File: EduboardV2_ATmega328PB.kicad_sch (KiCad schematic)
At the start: 25 parts, among them J1 EduboardV2 PCIE UP Board Conn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, SW1 K2-1102SP-C4SC-04, U2 ATMEGA328PB-AUR

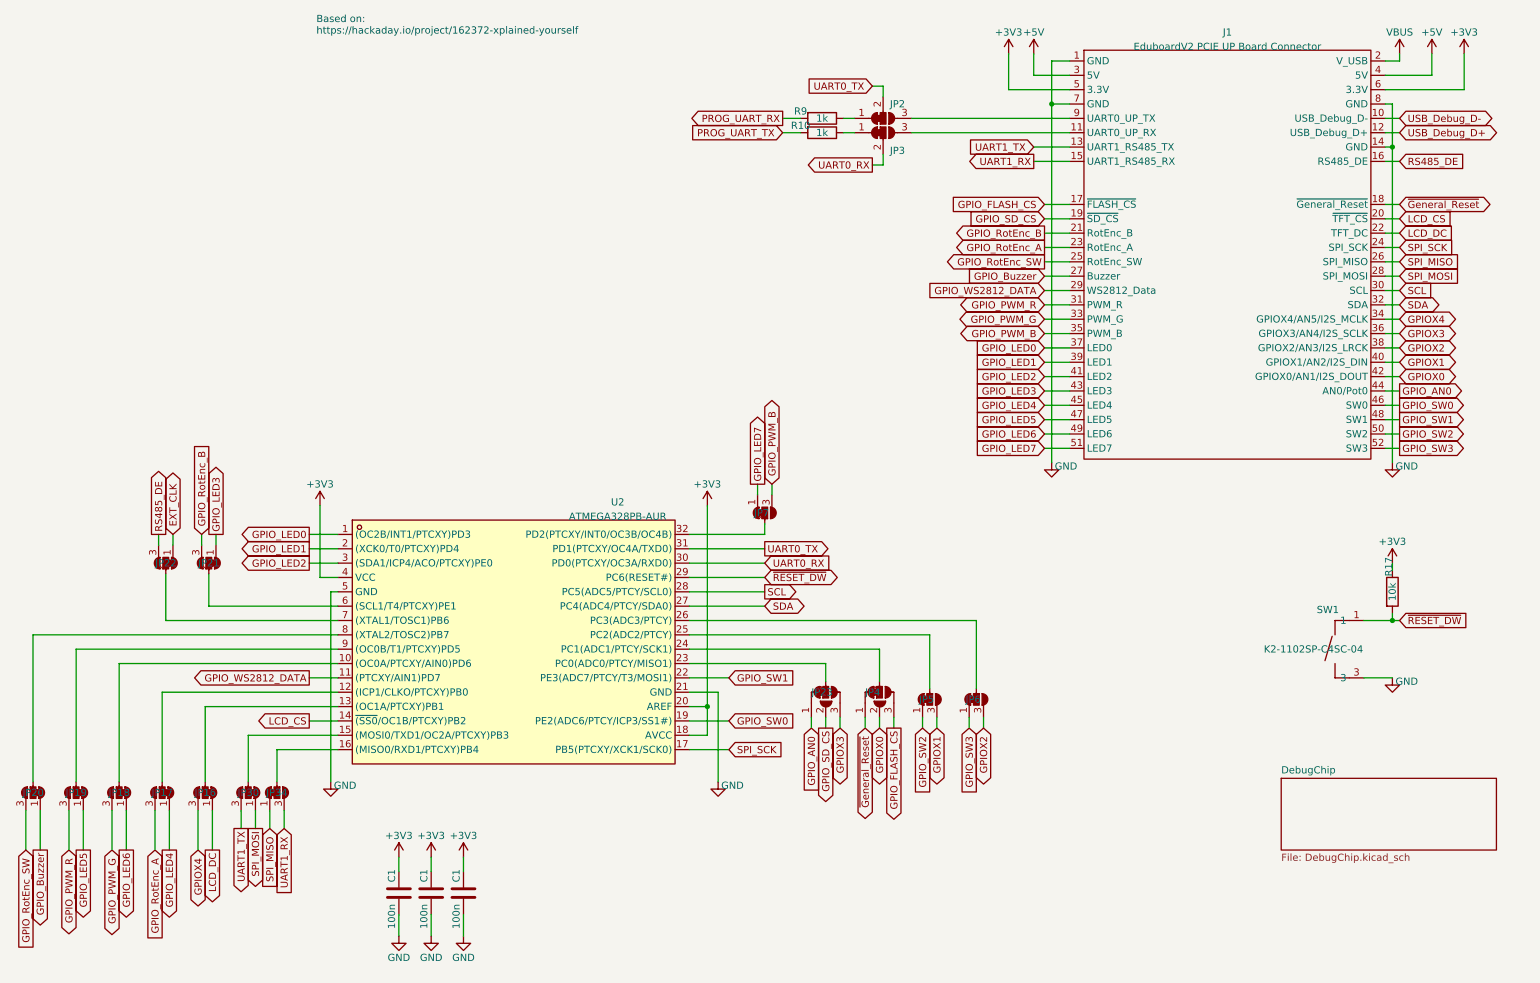
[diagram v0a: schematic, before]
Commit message: arrange parts and layout v1.1.
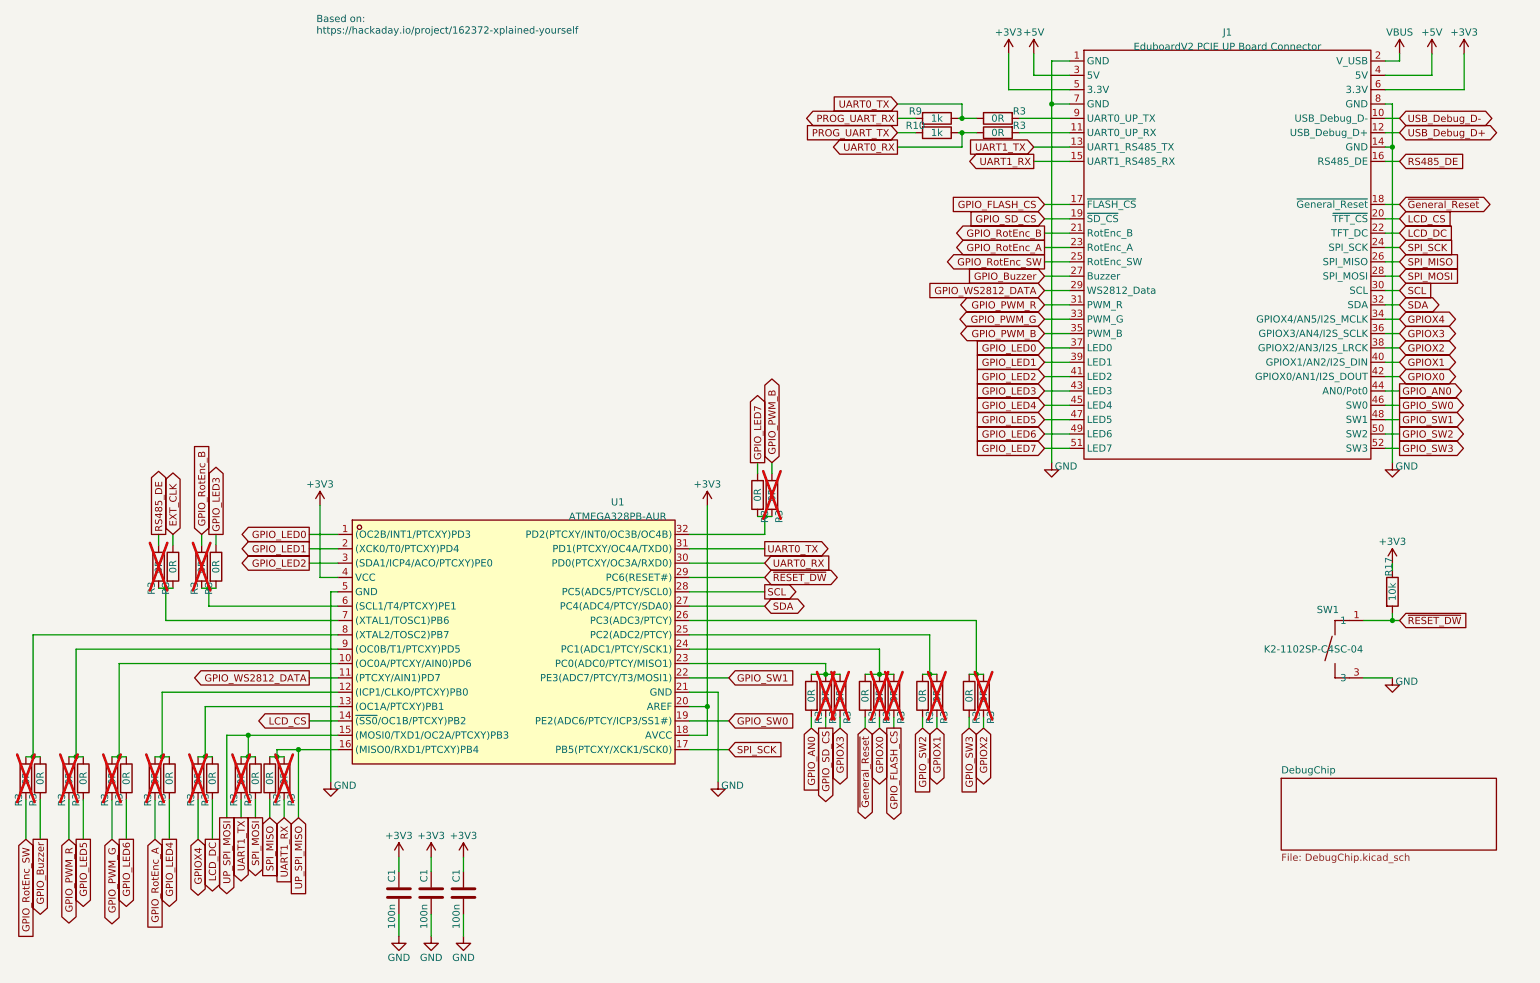
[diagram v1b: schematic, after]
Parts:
- removed JP16, JP17, JP18, JP19, JP20, JP21, JP22, JP30, JP34, JP5, JP6, JP7: SolderJumper_3_Bridged12, EduboardV2_kicadlib:SolderJumper_Small-3_bridged12, symbol EduboardV2_kicadlib:SolderJumper_Small_3_Bridged12
- removed JP2, JP3: SolderJumper_3_Bridged12, EduboardV2_kicadlib:SolderJumper_Small-3_bridged12, symbol Jumper:SolderJumper_3_Bridged12
- removed JP23, JP4: SolderJumper_3_Bridged12, EduboardV2_kicadlib:SolderJumper_Small-4_bridged14, symbol EduboardV2_kicadlib:SolderJumper_Small_4_Bridged14
- added R3 (x32): 0R, Resistor_SMD:R_0603_1608Metric, symbol Device:R
- renumbered U2 to U1
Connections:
- net EXT_CLK: now also R3.1
- net GPIOX0: now also R3.2
- net GPIOX1: now also R3.2
- net GPIOX2: now also R3.2
- net GPIOX3: now also R3.2
- net GPIOX4: now also R3.2
- net GPIO_AN0: now also R3.2
- net GPIO_Buzzer: now also R3.2
- net GPIO_FLASH_CS: now also R3.2
- net GPIO_LED3: now also R3.1
- net GPIO_LED4: now also R3.2
- net GPIO_LED5: now also R3.2
- net GPIO_LED6: now also R3.2
- net GPIO_LED7: now also R3.1
- net GPIO_PWM_B: now also R3.1
- net GPIO_PWM_G: now also R3.2
- net GPIO_PWM_R: now also R3.2
- net GPIO_RotEnc_A: now also R3.2
- net GPIO_RotEnc_B: now also R3.1
- net GPIO_RotEnc_SW: now also R3.2
- net GPIO_SD_CS: now also R3.2
- net GPIO_SW2: now also R3.2
- net GPIO_SW3: now also R3.2
- net LCD_DC: now also R3.2
- net RS485_DE: now also R3.1
- net SPI_MISO: now also R3.2
- net SPI_MOSI: now also R3.2
- net UART0_RX: now also R10.1, R3.1
- net UART0_TX: now also R9.1, R3.1
- net UART1_RX: now also R3.2
- net UART1_TX: now also R3.2
- net ~{General_Reset}: now also R3.2
- net UP_SPI_MOSI: now reaches U1.15 ((MOSI0/TXD1/OC2A/PTCXY)PB3)
- net UP_SPI_MOSI: now also R3.1, R3.1
- net at U1.24 (PC1(ADC1/PTCY/SCK1)): now also R3.1, R3.1, R3.1
- net at U1.12 ((ICP1/CLKO/PTCXY)PB0): now also R3.1, R3.1
- net at J1.9 (UART0_UP_TX): now also R3.2
- net at J1.11 (UART0_UP_RX): now also R3.2
- net at U1.26 (PC3(ADC3/PTCY)): now also R3.1, R3.1
- net at U1.32 (PD2(PTCXY/INT0/OC3B/OC4B)): now also R3.2, R3.2
- net at U1.10 ((OC0A/PTCXY/AIN0)PD6): now also R3.1, R3.1
- net at U1.13 ((OC1A/PTCXY)PB1): now also R3.1, R3.1
- net UP_SPI_MISO: now reaches U1.16 ((MISO0/RXD1/PTCXY)PB4)
- net UP_SPI_MISO: now also R3.1, R3.1
- net at U1.23 (PC0(ADC0/PTCY/MISO1)): now also R3.1, R3.1, R3.1
- net at U1.25 (PC2(ADC2/PTCY)): now also R3.1, R3.1
- net at U1.6 ((SCL1/T4/PTCXY)PE1): now also R3.2, R3.2
- net at U1.7 ((XTAL1/TOSC1)PB6): now also R3.2, R3.2
- net at U1.8 ((XTAL2/TOSC2)PB7): now also R3.1, R3.1
- net at U1.9 ((OC0B/T1/PTCXY)PD5): now also R3.1, R3.1
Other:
- moved on the sheet: R10, R9
